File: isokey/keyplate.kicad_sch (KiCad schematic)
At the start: 144 parts

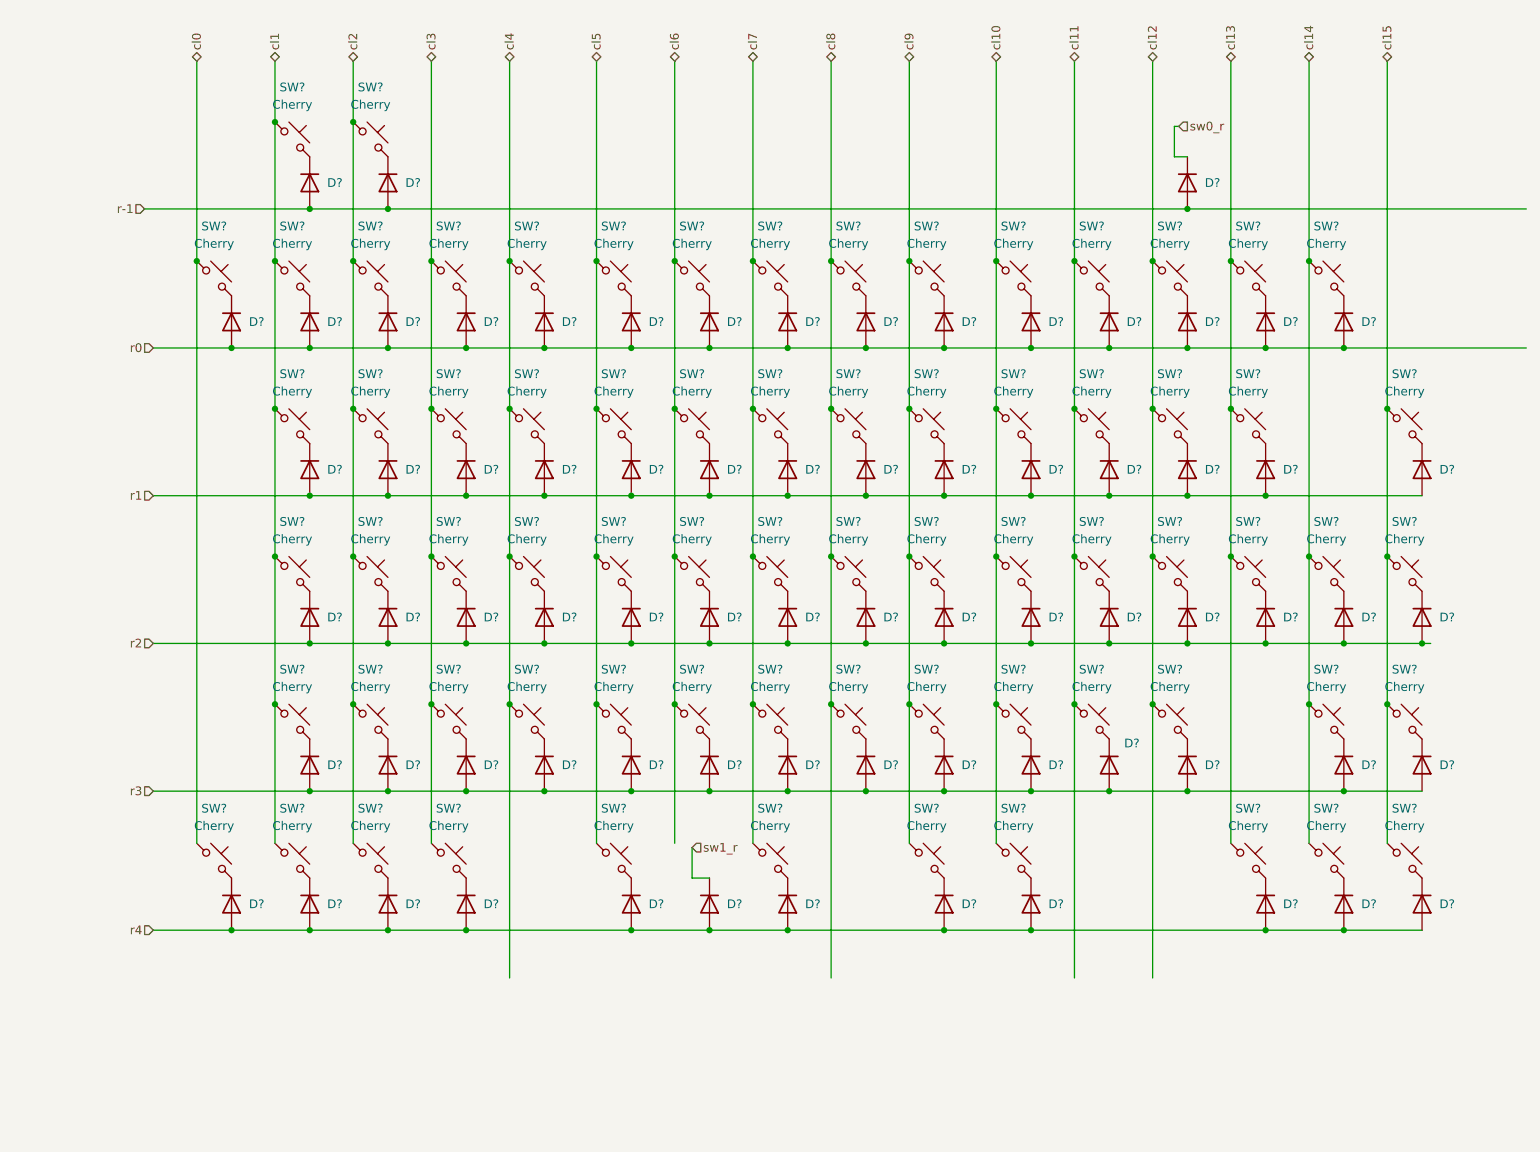
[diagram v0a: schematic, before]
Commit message: isokey: start splitting
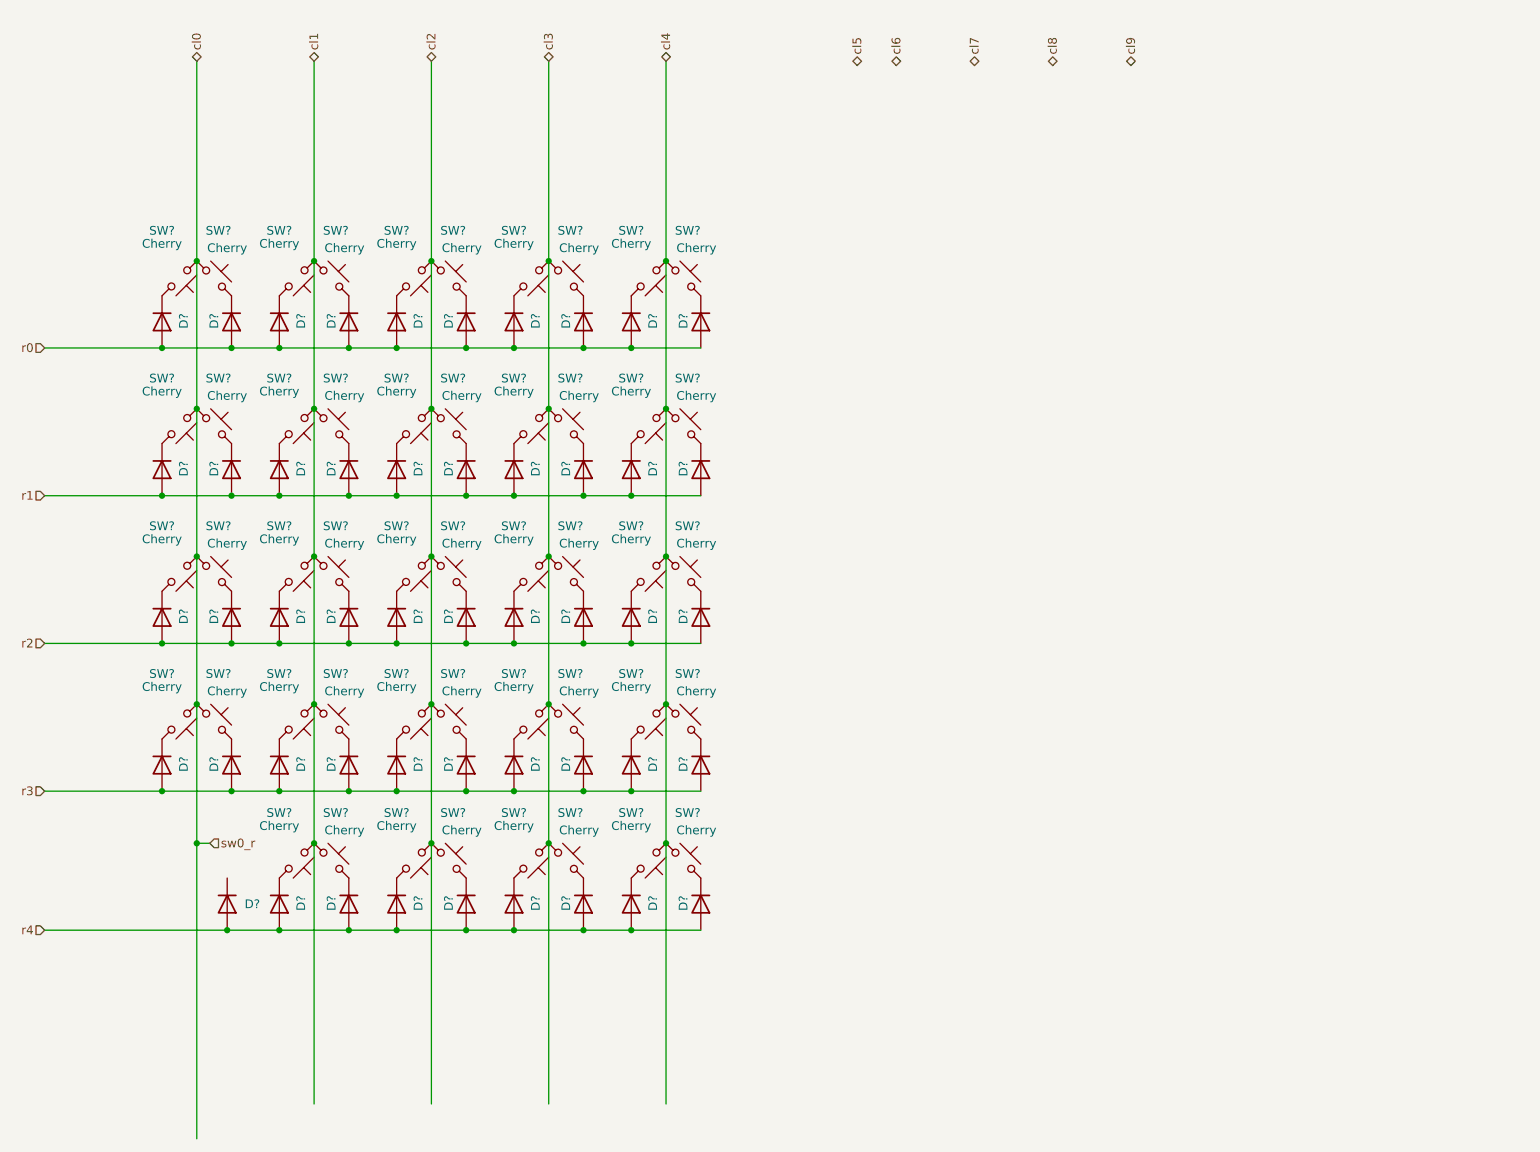
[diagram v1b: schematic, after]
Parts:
- removed D? (x72): 1N4448W, Diode_SMD:D_SOD-123, symbol Diode:1N4448W
- removed SW? (x70): Cherry, Button_Switch_Keyboard:Kailh_socket_MX_LED, symbol Switch:SW_Push_45deg
- added D? (x48): 1N4448W, Diode_SMD:D_SOD-123, symbol Diode:1N4448W
- added SW? (x47): Cherry, Button_Switch_Keyboard:Kailh_socket_MX_LED, symbol Switch:SW_Push_45deg
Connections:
- net cl0: now also SW?.1, SW?.1, SW?.1, SW?.2, SW?.2, SW?.2, SW?.2
- net cl1: now also SW?.1, SW?.1, SW?.1, SW?.1, SW?.1, SW?.2, SW?.2, SW?.2, SW?.2, SW?.2
- net cl2: now also SW?.1, SW?.1, SW?.1, SW?.1, SW?.1, SW?.2, SW?.2, SW?.2, SW?.2, SW?.2
- net cl3: now also SW?.1, SW?.1, SW?.1, SW?.1, SW?.1, SW?.2, SW?.2, SW?.2, SW?.2, SW?.2
- net cl4: now also SW?.1, SW?.1, SW?.1, SW?.1, SW?.1, SW?.2, SW?.2, SW?.2, SW?.2, SW?.2
- net r0: now also D?.2 (A), D?.2 (A), D?.2 (A), D?.2 (A), D?.2 (A), D?.2 (A), D?.2 (A), D?.2 (A), D?.2 (A)
- net r1: now also D?.2 (A), D?.2 (A), D?.2 (A), D?.2 (A), D?.2 (A), D?.2 (A), D?.2 (A), D?.2 (A), D?.2 (A), D?.2 (A)
- net r2: now also D?.2 (A), D?.2 (A), D?.2 (A), D?.2 (A), D?.2 (A), D?.2 (A), D?.2 (A), D?.2 (A), D?.2 (A), D?.2 (A)
- net r3: now also D?.2 (A), D?.2 (A), D?.2 (A), D?.2 (A), D?.2 (A), D?.2 (A), D?.2 (A), D?.2 (A), D?.2 (A), D?.2 (A)
- net r4: now also D?.2 (A), D?.2 (A), D?.2 (A), D?.2 (A), D?.2 (A), D?.2 (A), D?.2 (A), D?.2 (A), D?.2 (A)
- new net: D?.1 (K), SW?.2 (x23)
- new net: D?.1 (K), SW?.1 (x24)
